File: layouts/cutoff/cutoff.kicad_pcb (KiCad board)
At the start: 2 copper layers, 9 parts

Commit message: desktop push
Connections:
- C1 pad 2: C-1 -> C
- P1 pad 2: C -> C-1
- Q1 pad 3: C-1 -> C
- Q2 pad 5: C -> C-1
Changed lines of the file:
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@@
     (net 1 "K")
     (net 3 "SC_Sense")
-    (net 6 "C-1")
-    (net 8 "C")
+    (net 6 "C")
+    (net 8 "C-1")
     (net 9 "gnd")
     (net 12 "CUTOFF_GATE")
@@
             (drill 1.199896)
             (layers "*.Cu" "*.Mask")
-            (net 8 "C")
+            (net 8 "C-1")
         )
     )
@@
             (drill 0.9999979999999999)
             (layers "*.Cu" "*.Mask")
-            (net 6 "C-1")
+            (net 6 "C")
         )
         (pad "1" thru_hole circle
@@
             (size 1.25 0.7)
             (layers "F.Cu" "F.Paste" "F.Mask")
-            (net 6 "C-1")
+            (net 6 "C")
         )
     )
@@
                 )
             )
-            (net 8 "C")
+            (net 8 "C-1")
         )
         (pad "1" smd rect

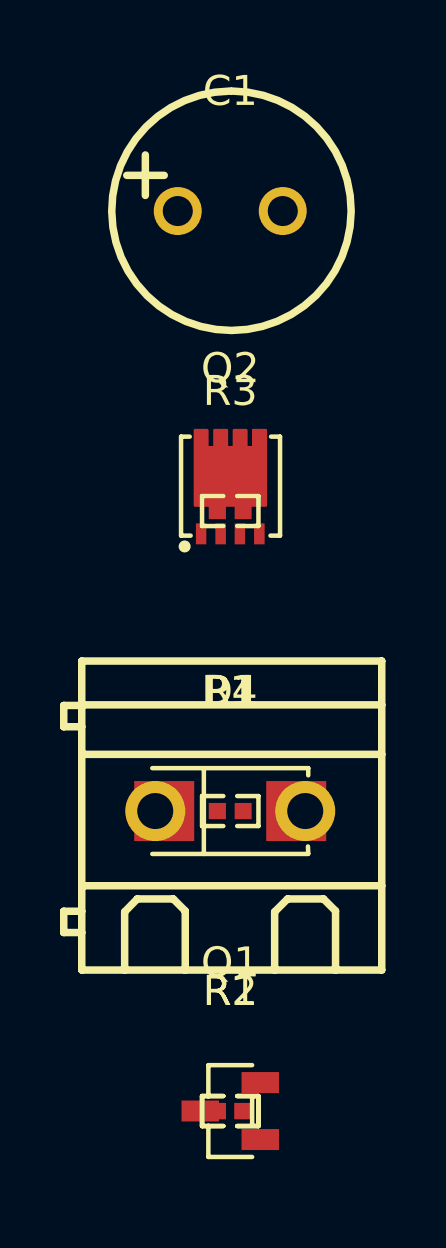
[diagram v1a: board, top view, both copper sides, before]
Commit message: im cooking
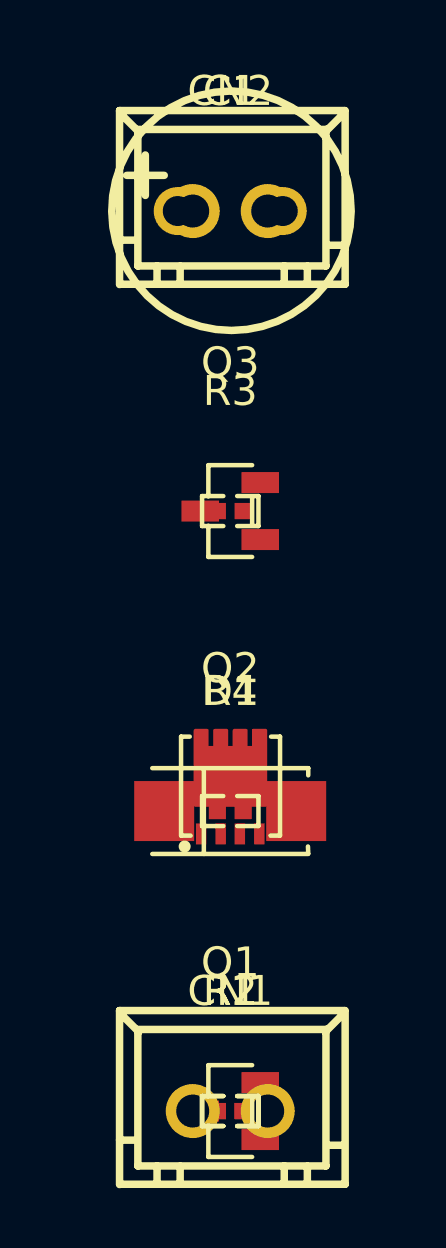
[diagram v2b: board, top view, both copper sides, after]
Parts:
- removed P1: , atopile:CONN-TH_2P-P5.00_WJ128V-5.0-2P-75f14f
- added CN1: , atopile:CONN-TH_XH-2A-b4a6f6, F.Cu at (0.00, 0.00)
- added CN2: , atopile:CONN-TH_XH-2A-b4a6f6, F.Cu at (0.00, -30.0)
- added Q3: , atopile:SOT-23-3_L2.9-W1.3-P1.90-LS2.4-BR-688f29, F.Cu at (0.00, -20.0)
- R1, R2, R3, R4: value 1kΩ ±1% 62.5mW -> 10kΩ ±1% 62.5mW
- moved Q2 10.0 mm to (0.00, -10.0)
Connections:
- net C renamed C-2

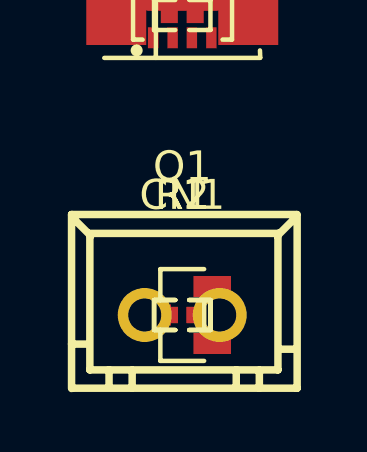
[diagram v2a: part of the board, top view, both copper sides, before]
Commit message: im cooking
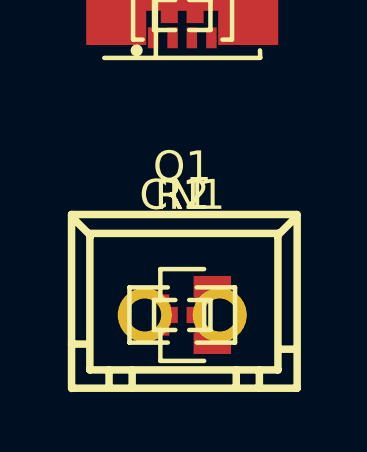
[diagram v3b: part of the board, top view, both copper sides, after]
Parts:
- R1: value 10kΩ ±1% 62.5mW -> 10kΩ ±1% 125mW; footprint atopile:R0402-56259e -> atopile:R0805-c79e8b
- R2, R3, R4: value 10kΩ ±1% 62.5mW -> 1kΩ ±1% 62.5mW
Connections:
- CN1 pad 2: C-1 -> C
- CN2 pad 2: C -> C-1
- Q2 pad 5: C-1 -> C
- Q3 pad 3: C -> C-1
